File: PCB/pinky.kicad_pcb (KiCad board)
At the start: 2 copper layers, 133.5 x 87.7 mm, 54 parts, among them SW10 Switch, SW11 Switch, SW12 Switch, SW13 Switch, SW14 Switch, SW15 Switch, SW16 Switch, SW17 Switch, SW18 Switch, SW2 Switch, SW3 Switch, SW5 Switch, SW6 Switch, SW7 Switch, SW8 Switch, SW9 Switch, U1 nice!nano

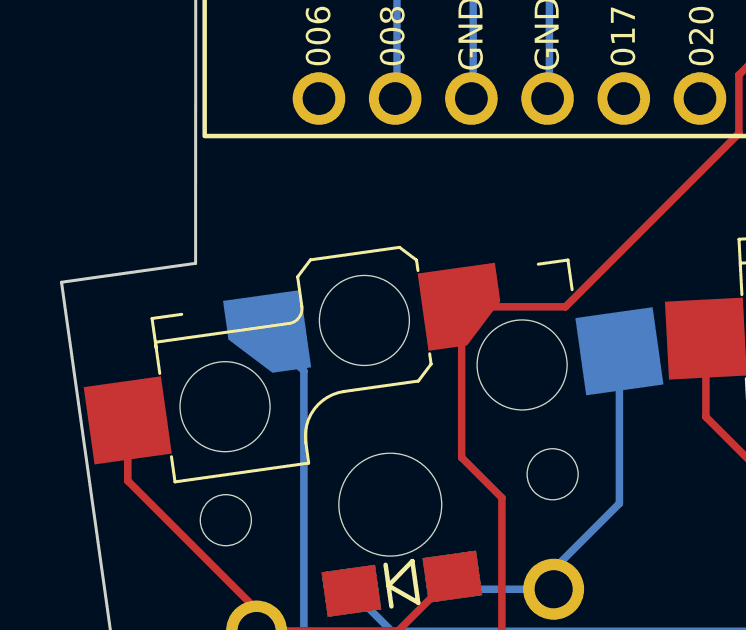
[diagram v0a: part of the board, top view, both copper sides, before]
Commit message: Footprints and scheme update
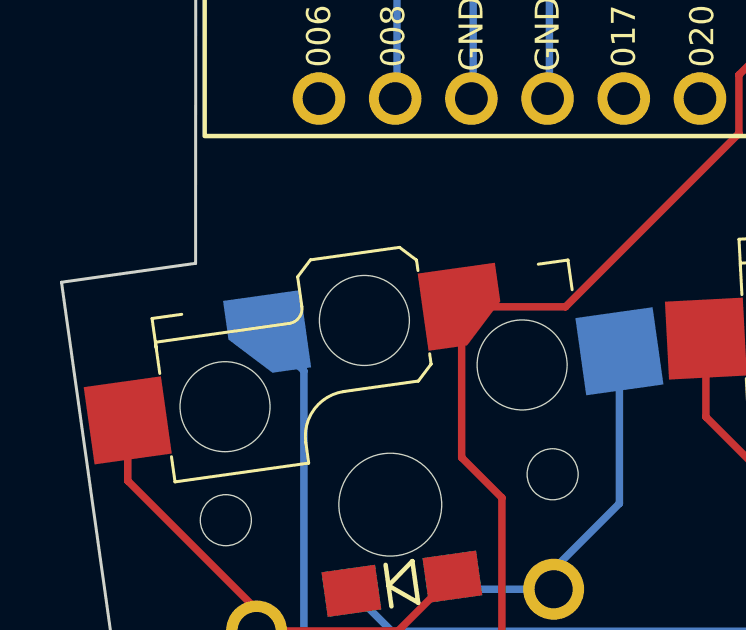
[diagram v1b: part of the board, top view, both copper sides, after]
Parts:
- JP2, JP3, JP4: value Jumper -> SDA
